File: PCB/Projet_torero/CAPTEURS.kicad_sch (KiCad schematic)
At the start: 7 parts, among them J401 Conn_01x08, J402 Conn_02x02_Counter_Clockwise, U401 ADXL343

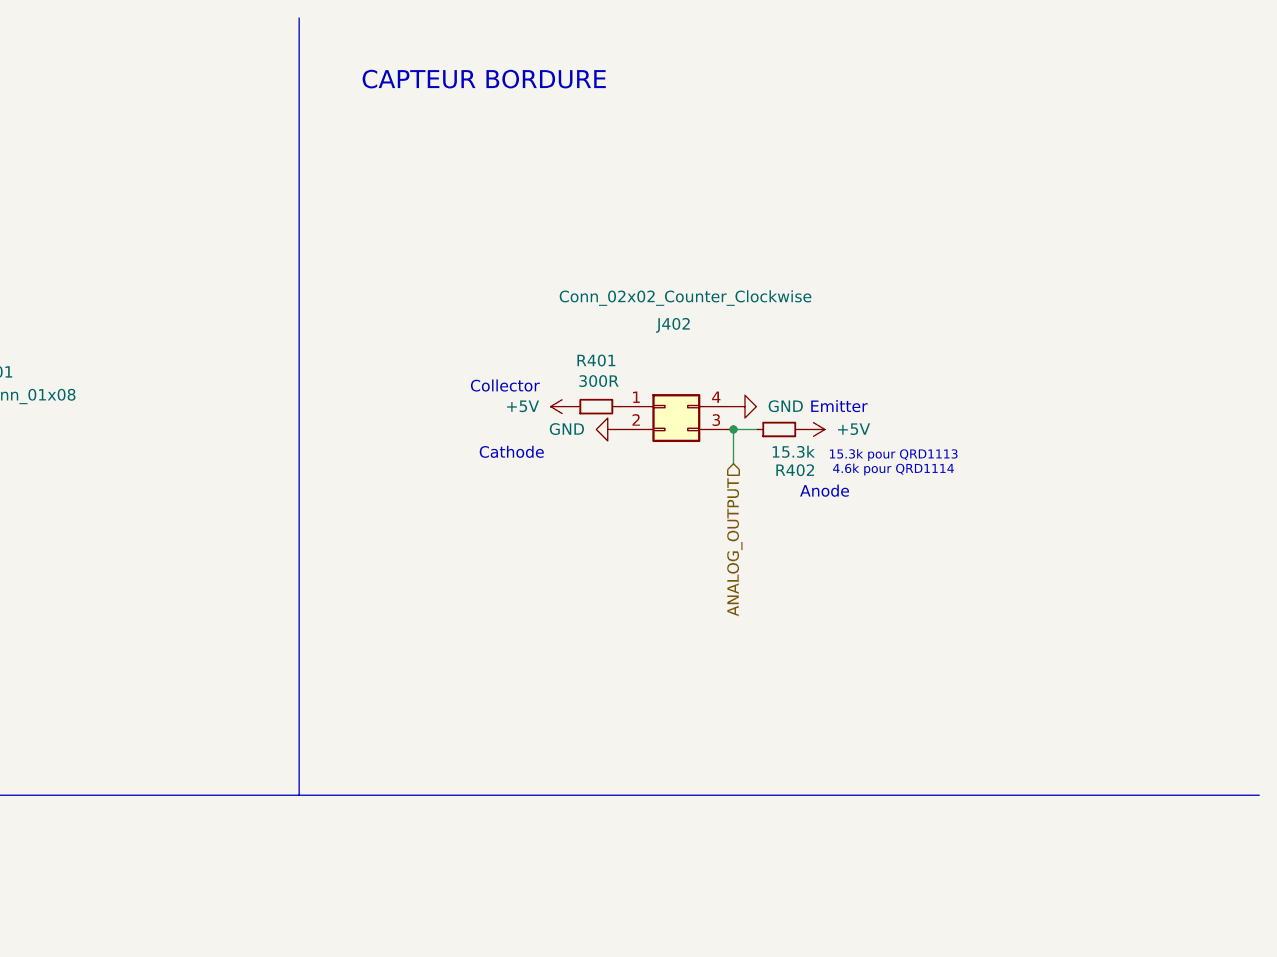
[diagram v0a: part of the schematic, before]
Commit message: modif kicad capteur
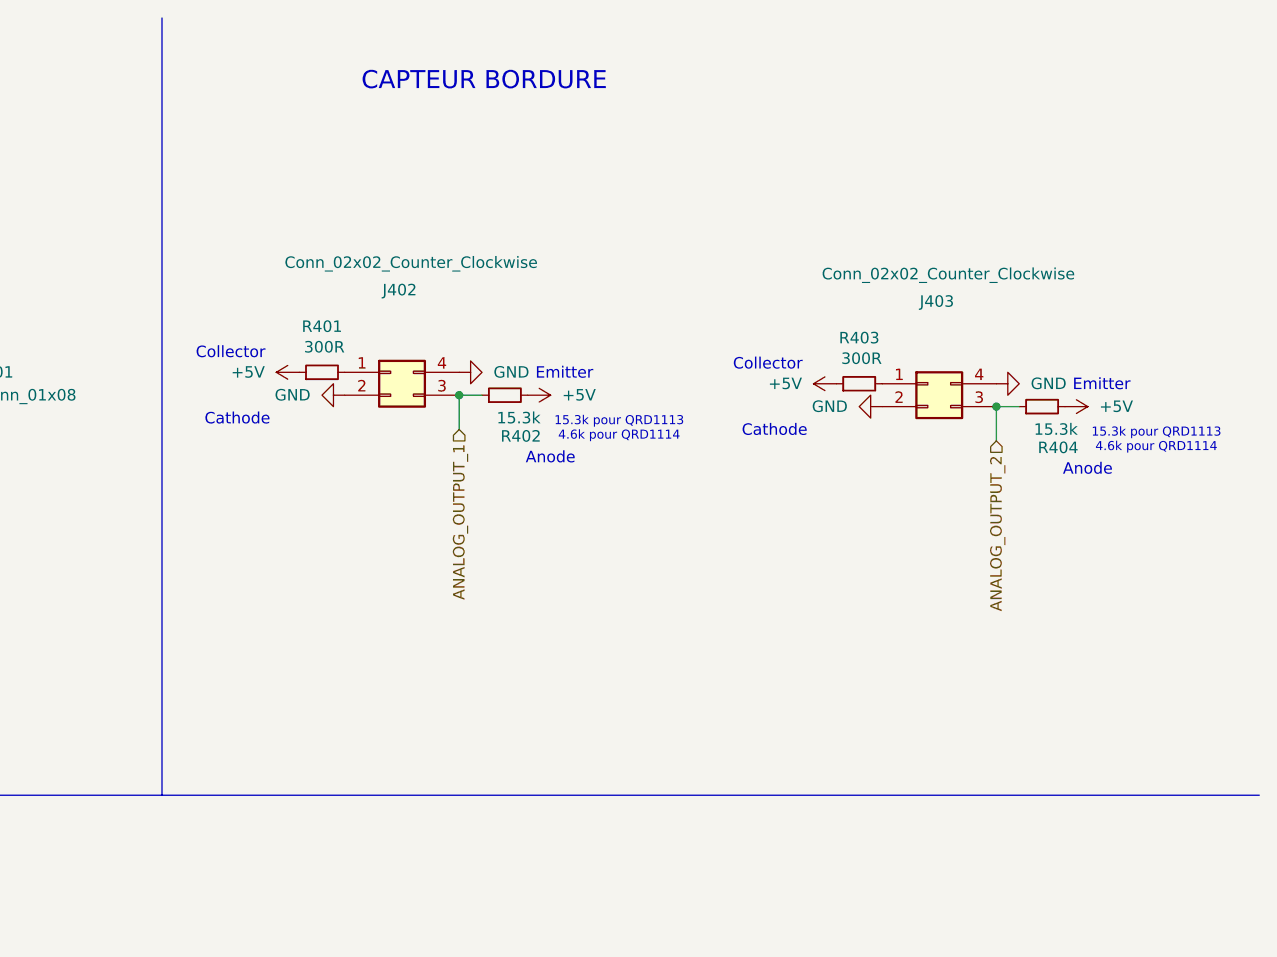
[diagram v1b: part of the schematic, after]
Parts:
- added J403: Conn_02x02_Counter_Clockwise, symbol Connector_Generic:Conn_02x02_Counter_Clockwise
- added R403: 300R, symbol Device:R_Small
- added R404: 15.3k, symbol Device:R_Small
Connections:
- net +5V: now also R403.1, R404.2
- net GND: now also J403.2 (Pin_2), J403.4 (Pin_4)
- net ANALOG_OUTPUT renamed ANALOG_OUTPUT_1
- new net: J403.1 (Pin_1), R403.2
- new net ANALOG_OUTPUT_2: J403.3 (Pin_3), R404.1
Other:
- moved on the sheet: J402, R401, R402
